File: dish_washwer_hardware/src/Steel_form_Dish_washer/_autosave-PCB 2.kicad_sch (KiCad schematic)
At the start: 25 parts, among them J16 SCREEN CONNECTOR, J18 Conn_02x07_Odd_Even, J8 Conn_01x10_Male, U15 TXS0108EPW, U16 EAST1616RGBA8, U17 EAST1616RGBA8, U18 MPR121QR2

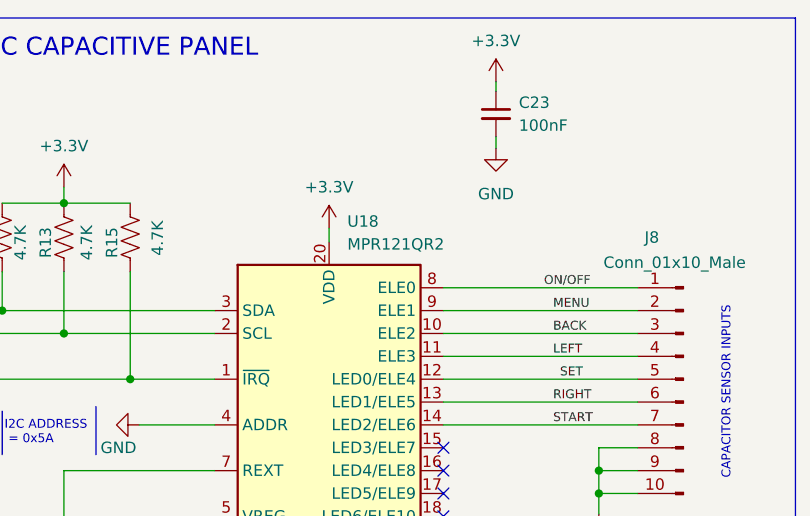
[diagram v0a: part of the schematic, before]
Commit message: updated firmware
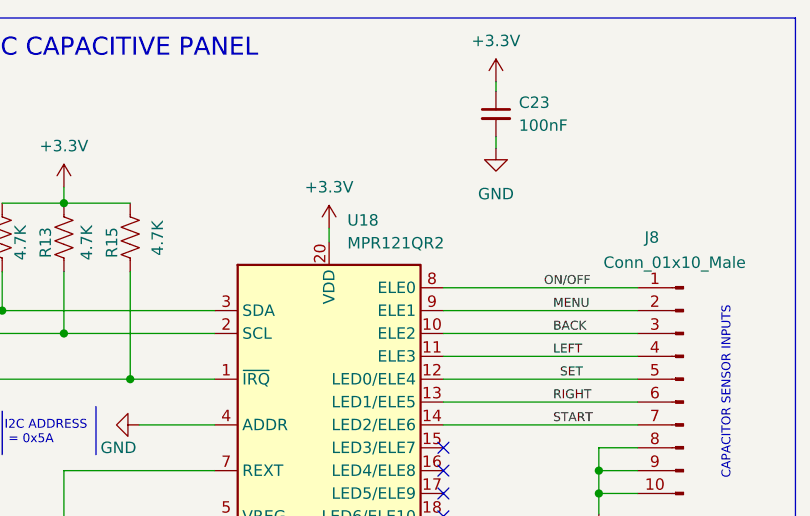
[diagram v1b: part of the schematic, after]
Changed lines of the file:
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@@
   (symbol (lib_id "Sensor_Touch:MPR121QR2") (at 224.79 62.103 0) (unit 1)
     (in_bom yes) (on_board yes) (fields_autoplaced)
-    (property "Reference" "U18" (id 0) (at 226.8094 39.497 0)
+    (property "Reference" "U18" (id 0) (at 226.8094 39.37 0)
       (effects (font (size 1.27 1.27)) (justify left))
     )
-    (property "Value" "MPR121QR2" (id 1) (at 226.8094 42.037 0)
+    (property "Value" "MPR121QR2" (id 1) (at 226.8094 41.91 0)
       (effects (font (size 1.27 1.27)) (justify left))
     )
